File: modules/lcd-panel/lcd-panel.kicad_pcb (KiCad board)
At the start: 4 copper layers, 40 x 91.4 mm, 10 parts, among them J1 5051100692, J2 5051104091, U1 LP8556SQ-E09/NOPB

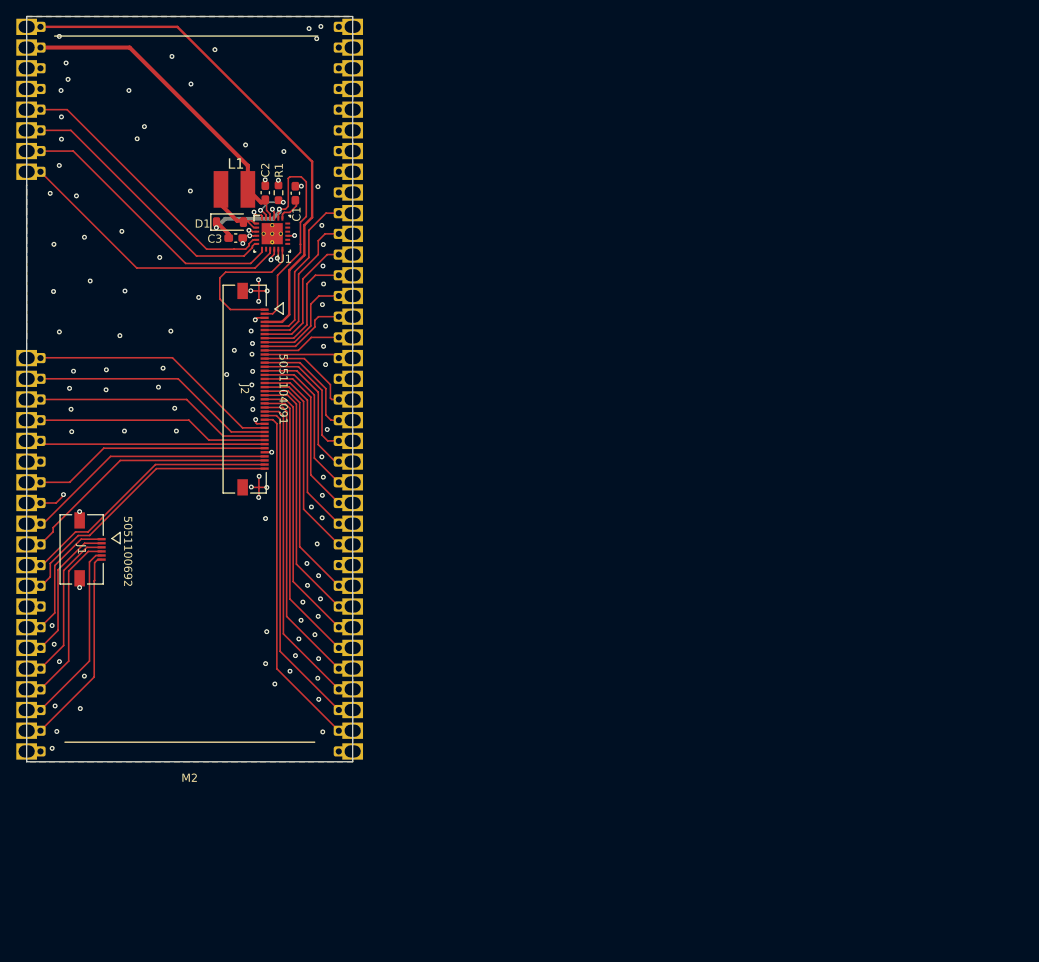
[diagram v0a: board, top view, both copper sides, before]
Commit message: Routing
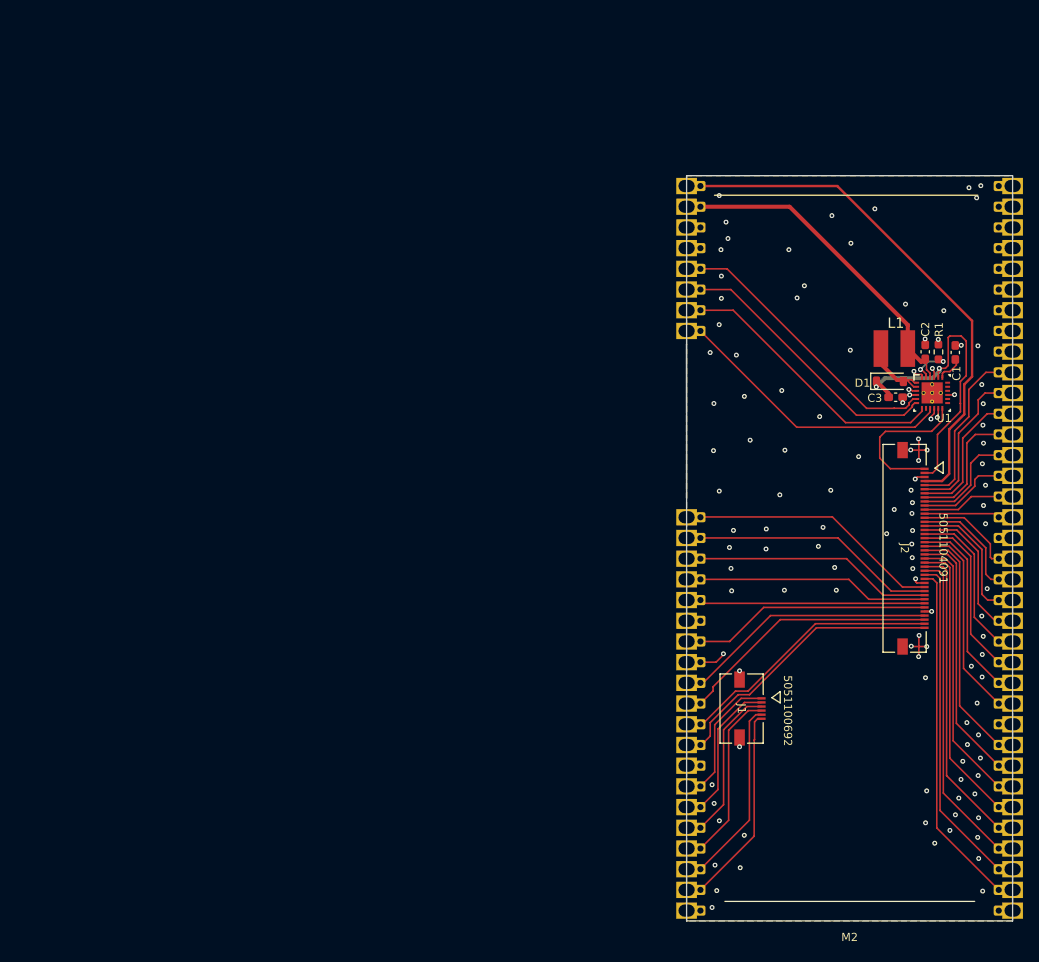
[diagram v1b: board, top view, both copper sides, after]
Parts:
- moved C2 83.3 mm to (198.6, 91.3)
- moved J1 83.3 mm to (176.1, 135.1)
- moved U1 83.3 mm to (199.5, 96.4)
- moved C1 83.3 mm to (202.3, 91.4)
- moved D1 83.3 mm to (194.3, 94.9)
- moved J2 83.3 mm to (196.1, 115.4)
- moved M2 83.3 mm to (189.4, 115.4)
- moved C3 83.3 mm to (195.0, 96.9)
- moved L1 83.3 mm to (194.9, 90.9)
- moved R1 83.3 mm to (200.3, 91.3)
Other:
- board text added: "LCD"
